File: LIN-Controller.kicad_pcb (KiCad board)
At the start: 2 copper layers, 40.6 x 80.3 mm, 56 parts, among them CON1 BARREL_JACK, J1 SWD_HEADER, J2 1881451_LIN, M2Hole VAL**, SW1 GP12MCBE, SW2 THUMBWHEEL, SW3 TL9210, SW4 TL9210, SW5 TL9210, SW6 TL9210, U1 2SC5662, U2 SAMC21E-A, U3 TPS7133QD, U4 2SC5662, U5 2SC5662, U6 2SC5662, U7 ATA663211

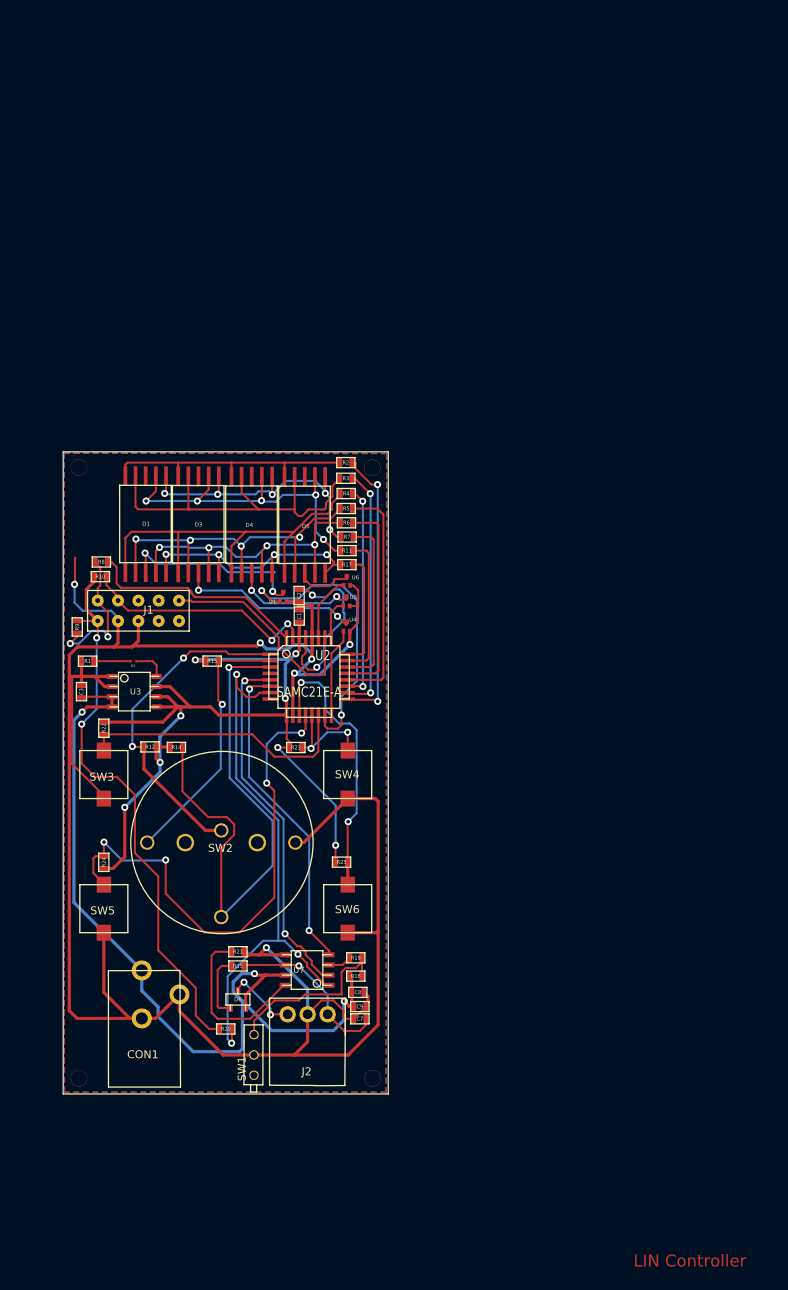
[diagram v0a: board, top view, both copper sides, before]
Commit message: Added files via upload
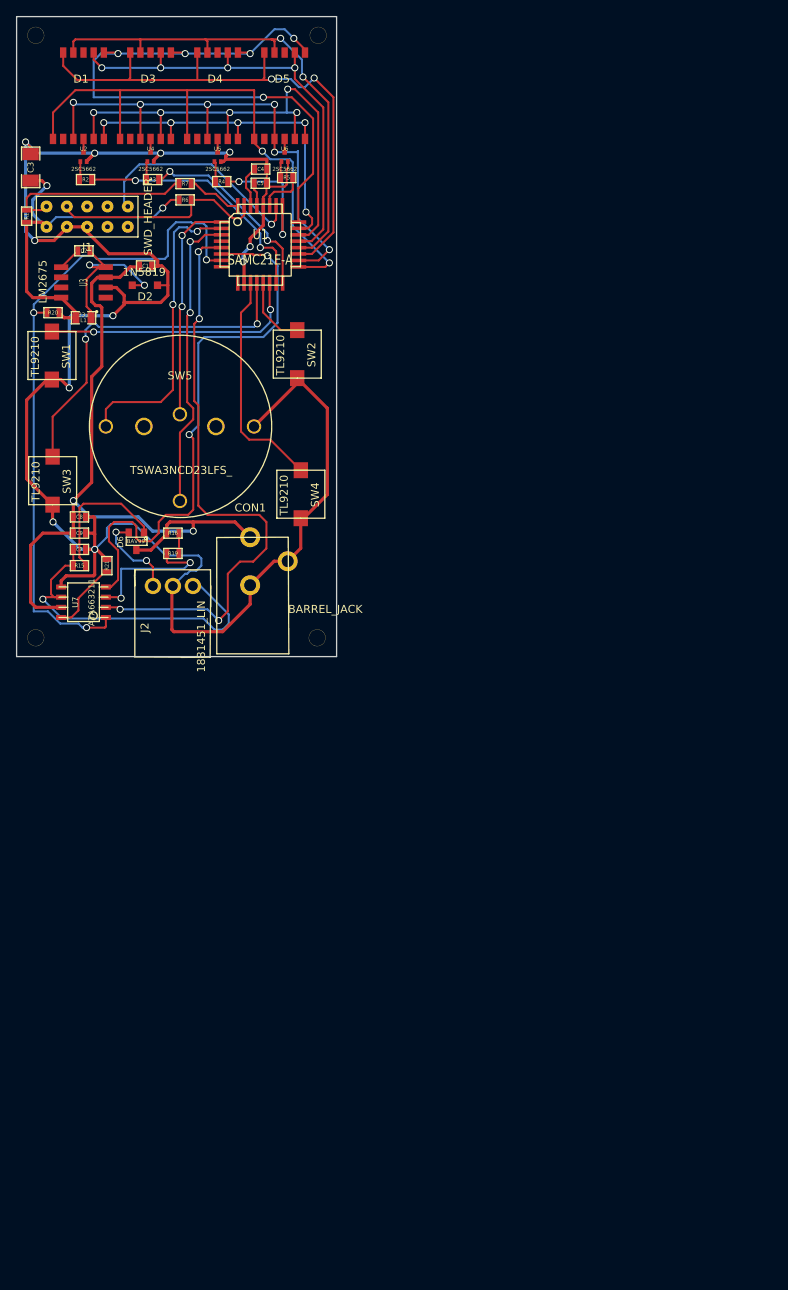
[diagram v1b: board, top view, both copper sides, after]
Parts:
- removed M2Hole (x4): VAL**, M2Hole
- removed R10, R9: 10K, SM0603
- removed R11, R17: 200, SM0603
- removed R12, R13, R14, R22, R23, R24, R25: 4K7, SM0603
- removed R8: 22R, SM0603
- removed SW6: TL9210, TL9210
- added C4: 0.1u, SM0603, F.Cu at (140.5, 54.1)
- added C5: 0.1u, SM0603, F.Cu at (140.5, 55.8)
- added L1: 33u, SM0805, F.Cu at (118.4, 72.6)
- added REF**: 1pin, Connect:1pin, F.Cu at (147.6, 112.6)
- added REF**: 1pin, Connect:1pin, F.Cu at (112.4, 112.6)
- added REF**: 1pin, Connect:1pin, F.Cu at (112.4, 37.3)
- added REF**: 1pin, Connect:1pin, F.Cu at (147.7, 37.3)
- C1: value 0.1u -> 47u
- C3: value 0.1u -> 100u; footprint SM0603 -> SM1206
- D1, D3, D4, D5: value 7_SEGMENT_DISPLAY -> HDSM-283L; footprint 511-1570-2-ND -> HDSM-283
- D2: value XZMYR155W -> 1N5819; footprint XZMYR155W -> SOD123
- D6: footprint sot23 -> SOT23
- R1, R6: value 200 -> 10K
- R2, R3, R4, R5: value 200 -> 330R
- R7: value 200 -> 22R
- SW1: value GP12MCBE -> TL9210; footprint GP12MCBE -> TL9210
- SW2: value THUMBWHEEL -> TL9210; footprint TSWA3NCD23LFS -> TL9210
- SW5: value TL9210 -> TSWA3NCD23LFS_; footprint TL9210 -> TSWA3NCD23LFS
- U1: value 2SC5662 -> SAMC21E-A; footprint SOT723 -> TQFP32
- U2: value SAMC21E-A -> 2SC5662; footprint TQFP32 -> SOT723
- U3: value TPS7133QD -> LM2675; footprint so-8 -> SOIC8-narrow
- moved R20 92.1 mm to (114.6, 72.0), turned to 180 degrees
- moved SW1 88.1 mm to (114.4, 80.4), turned to 270 degrees
- moved U2 71.0 mm to (118.4, 52.3)
- moved C8 68.9 mm to (117.9, 97.5)
- moved C9 68.8 mm to (117.9, 99.6)
- moved C7 68.3 mm to (117.9, 101.6), turned to 0 degrees
- moved C3 65.8 mm to (111.8, 53.8)
- moved U4 63.6 mm to (126.7, 52.3)
- moved R16 59.9 mm to (129.5, 99.6)
- moved SW2 58.8 mm to (145.1, 80.2), turned to 270 degrees
- moved D6 58.7 mm to (125.0, 100.6), turned to 180 degrees
- moved SW5 58.1 mm to (130.4, 86.2), turned to 0 degrees
- moved U5 57.8 mm to (135.1, 52.3)
- moved R1 56.1 mm to (111.3, 59.9), turned to 90 degrees
- moved J2 56.1 mm to (129.5, 106.2)
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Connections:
- C1 pad 1: 3V3 -> VsLIN
- C2 pad 1: N-0000047 -> Net-(C2-Pad1)
- C2 pad 2: GND -> Net-(C2-Pad2)
- C3 pad 1: VsLIN -> 3V3
- D1 pad 1: N-0000055 -> /DIS'g'
- D1 pad 10: N-0000054 -> /DIS'd'
- D1 pad 2: N-0000056 -> Net-(D1-Pad2)
- D1 pad 3: N-000006 -> /DIS'f'
- D1 pad 4: N-0000057 -> (no net)
- D1 pad 5: N-0000032 -> /DIS'b'
- D1 pad 6: N-0000024 -> /DIS'a'
- D1 pad 7: N-0000018 -> /DIS'.'
- D1 pad 8: (no net) -> /DIS'c'
- D1 pad 9: N-0000058 -> Net-(D1-Pad9)
- D2 pad 1: N-0000027 -> GND
- D2 pad 2: N-0000050 -> Net-(C2-Pad2)
- D3 pad 1: N-0000055 -> /DIS'g'
- D3 pad 10: N-0000054 -> /DIS'd'
- D3 pad 2: N-0000056 -> Net-(D3-Pad2)
- D3 pad 3: N-000004 -> /DIS'f'
- D3 pad 4: N-0000057 -> (no net)
- D3 pad 5: N-0000032 -> /DIS'b'
- D3 pad 6: N-0000024 -> /DIS'a'
- D3 pad 7: N-0000018 -> /DIS'.'
- D3 pad 8: (no net) -> /DIS'c'
- D3 pad 9: N-0000058 -> Net-(D3-Pad9)
- D4 pad 1: N-0000055 -> /DIS'g'
- D4 pad 10: N-0000054 -> /DIS'd'
- D4 pad 2: N-0000056 -> Net-(D4-Pad2)
- D4 pad 3: N-000007 -> /DIS'f'
- D4 pad 4: N-0000057 -> (no net)
- D4 pad 5: N-0000032 -> /DIS'b'
- D4 pad 6: N-0000024 -> /DIS'a'
- D4 pad 7: N-0000018 -> /DIS'.'
- D4 pad 8: (no net) -> /DIS'c'
- D4 pad 9: N-0000058 -> Net-(D4-Pad9)
- D5 pad 1: N-0000055 -> /DIS'g'
- D5 pad 10: N-0000054 -> /DIS'd'
- D5 pad 2: N-0000056 -> Net-(D5-Pad2)
- D5 pad 3: N-000001 -> /DIS'f'
- D5 pad 4: N-0000057 -> (no net)
- D5 pad 5: N-0000032 -> /DIS'b'
- D5 pad 6: N-0000024 -> /DIS'a'
- D5 pad 7: N-0000018 -> /DIS'.'
- D5 pad 8: (no net) -> /DIS'c'
- D5 pad 9: N-0000058 -> Net-(D5-Pad9)
- J1 pad 1: Vcc -> 3V3
- J1 pad 10: N-0000044 -> Net-(J1-Pad10)
- J1 pad 2: N-0000038 -> Net-(J1-Pad2)
- J1 pad 4: N-0000042 -> Net-(J1-Pad4)
- J1 pad 6: (no net) -> Net-(J1-Pad6)
- J1 pad 8: (no net) -> Net-(J1-Pad8)
- J1 pad 9: (no net) -> Net-(J1-Pad9)
- R1 pad 1: GND -> 3V3
- R1 pad 2: N-0000050 -> Net-(J1-Pad2)
- R16 pad 2: N-000008 -> Net-(R16-Pad2)
- R19 pad 1: N-000008 -> Net-(R16-Pad2)
- R2 pad 1: N-0000054 -> /DS3
- R2 pad 2: N-0000026 -> Net-(R2-Pad2)
- R20 pad 1: Vcc -> 3V3
- R20 pad 2: N-0000033 -> /RXD
- R3 pad 1: N-0000058 -> /DS2
- R3 pad 2: N-0000020 -> Net-(R3-Pad2)
- R4 pad 1: N-0000055 -> /DS1
- R4 pad 2: N-0000021 -> Net-(R4-Pad2)
- R5 pad 1: N-0000056 -> /DS0
- R5 pad 2: N-0000019 -> Net-(R5-Pad2)
- R6 pad 1: N-0000057 -> 3V3
- R6 pad 2: N-0000022 -> Net-(J1-Pad4)
- R7 pad 1: N-0000024 -> Net-(R7-Pad1)
- R7 pad 2: N-0000023 -> Net-(J1-Pad2)
- SW1 pad 1: (no net) -> GND
- SW1 pad 2: GND -> /PB0
- SW2 pad 1: N-0000034 -> GND
- SW2 pad 2: N-0000036 -> /PB1
- SW3 pad 1: N-0000015 -> GND
- SW3 pad 2: GND -> /PB2
- SW4 pad 1: N-0000014 -> GND
- SW4 pad 2: GND -> /PB3
- SW5 pad 1: N-0000030 -> /TWA
- SW5 pad 2: GND -> /TWB
- U1 pad 1: N-000002 -> /TWC
- U1 pad 2: GND -> /TWA
- U1 pad 3: N-000006 -> /TWB
- U2 pad 1: N-0000037 -> Net-(R2-Pad2)
- U2 pad 2: N-0000034 -> GND
- U2 pad 3: N-0000036 -> Net-(D1-Pad3)
- U3 pad 1: GND -> Net-(C2-Pad1)
- U3 pad 2: GND -> Net-(U3-Pad2)
- U3 pad 3: VsLIN -> Net-(U3-Pad3)
- U3 pad 4: VsLIN -> 3V3
- U3 pad 5: 3V3 -> Net-(U3-Pad5)
- U3 pad 6: 3V3 -> GND
- U3 pad 7: 3V3 -> VsLIN
- U3 pad 8: N-0000027 -> Net-(C2-Pad2)
- U4 pad 1: N-000003 -> Net-(R3-Pad2)
- U4 pad 3: N-000004 -> Net-(D3-Pad3)
- U5 pad 1: N-0000012 -> Net-(R4-Pad2)
- U5 pad 3: N-000007 -> Net-(D4-Pad3)
- U6 pad 1: N-0000013 -> Net-(R5-Pad2)
- U6 pad 3: N-000001 -> Net-(D5-Pad3)
- U7 pad 1: N-0000033 -> /RXD
- U7 pad 2: N-0000011 -> /EN
- U7 pad 4: N-0000016 -> /TXD
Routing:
- net /RXD: track 0.00 -> 85.4 mm, vias 0 -> 3
- net /DIS'.': track 0.00 -> 81.5 mm, vias 0 -> 5
- net /EN: track 0.00 -> 75.3 mm, vias 0 -> 4
- net /DIS'g': track 0.00 -> 72.8 mm, vias 0 -> 2
- net /TXD: track 0.00 -> 71.3 mm, vias 0 -> 2
- net /DIS'e': track 0.00 -> 71.0 mm, vias 0 -> 2
- net Vcc: track 70.5 -> 0.00 mm, vias 2 -> 0
- net N-0000033: track 69.7 -> 0.00 mm, vias 3 -> 0
- net N-0000036: track 67.3 -> 0.00 mm, vias 1 -> 0
- net /DIS'f': track 0.00 -> 65.8 mm, vias 0 -> 6
- net N-0000030: track 64.3 -> 0.00 mm, vias 4 -> 0
- net 3V3: track 112.7 -> 48.6 mm, vias 8 -> 2
- net /DIS'd': track 0.00 -> 63.9 mm, vias 0 -> 2
- net /DIS'b': track 0.00 -> 63.9 mm, vias 0 -> 5
- net /DIS'c': track 0.00 -> 57.6 mm, vias 0 -> 4
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- removed copper zone on B.Cu, net GND
- removed copper zone on F.Cu, net GND
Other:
- board size 40.6 x 80.3 mm -> 40 x 80 mm
- rule pad_to_mask_clearance: 0 -> 0.2
- board text removed: "LIN Controller"
